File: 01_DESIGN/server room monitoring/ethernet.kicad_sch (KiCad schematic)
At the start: 38 parts, among them J6 HR911105A, U5 W5500, Y1 25 MHz

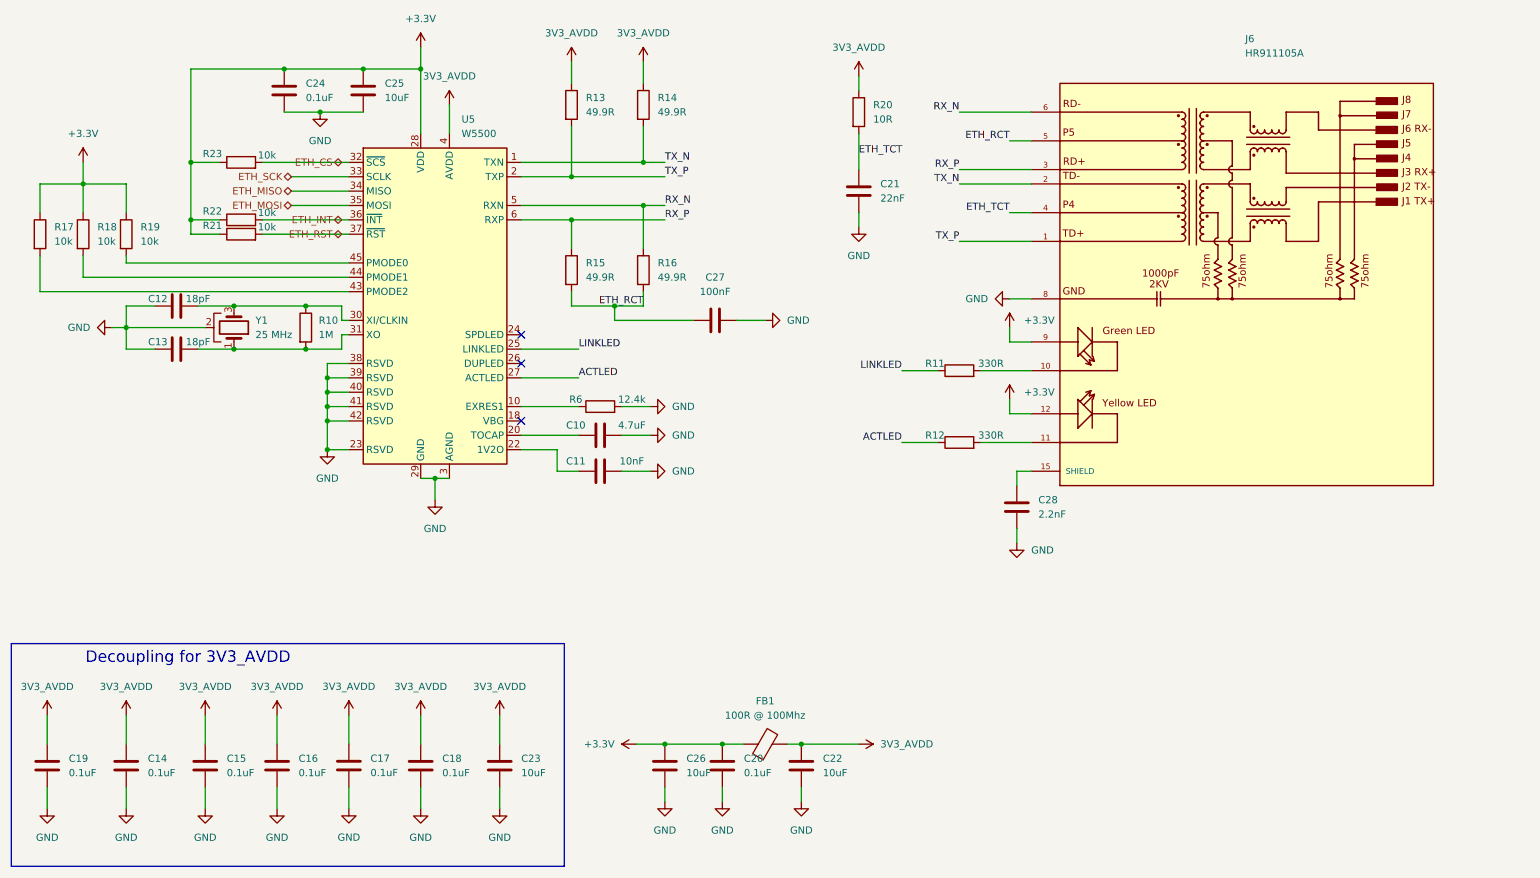
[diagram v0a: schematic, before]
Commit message: Update project files
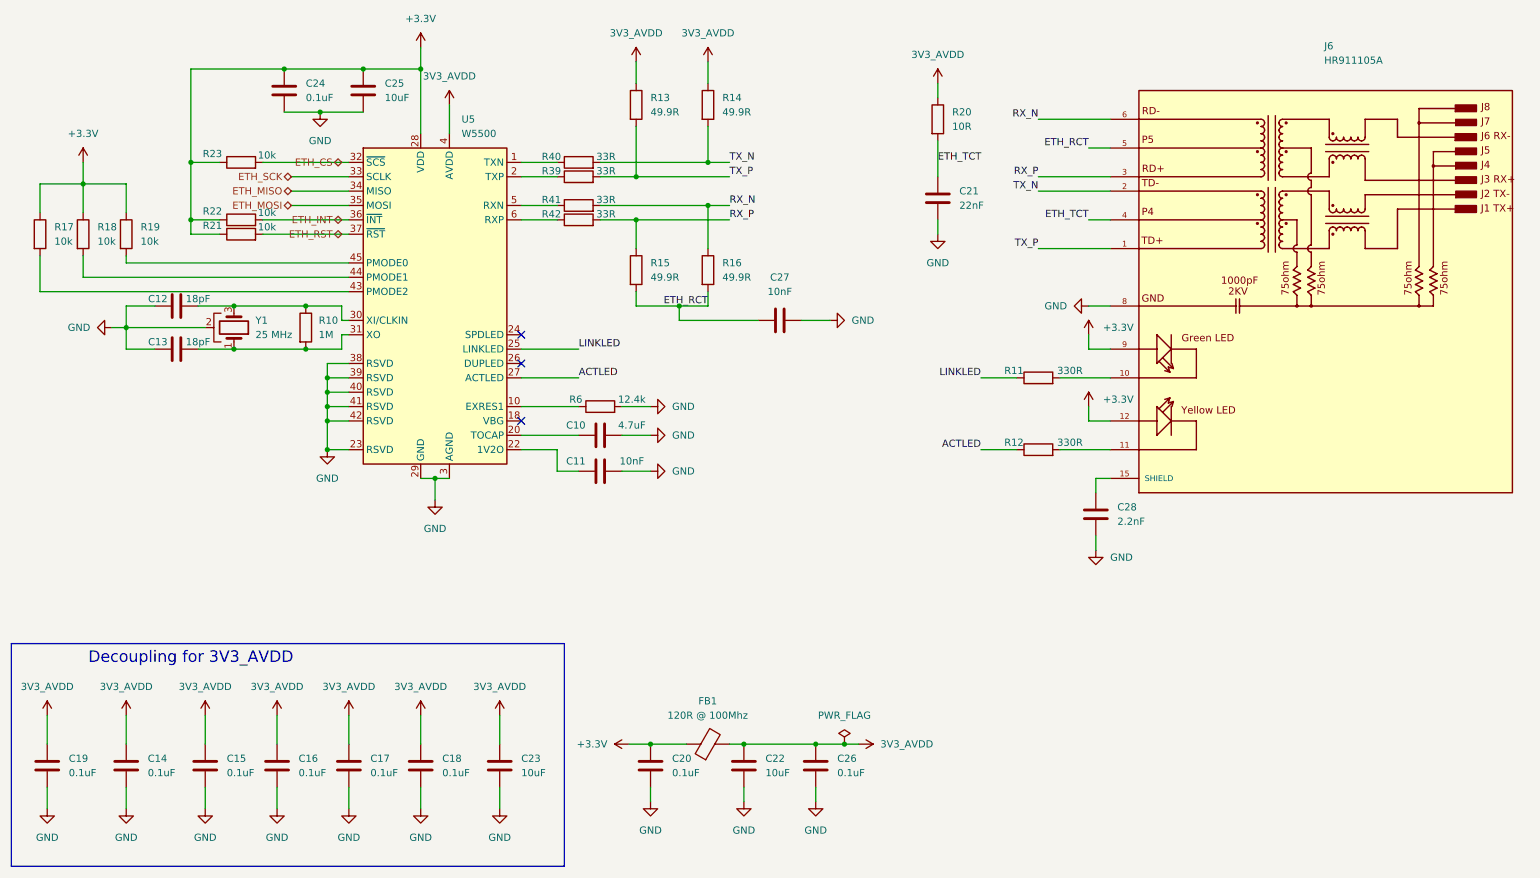
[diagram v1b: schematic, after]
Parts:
- added R39, R40, R41, R42: 33R, Resistor_SMD:R_0805_2012Metric, symbol Device:R
- C10, C11, C12, C13, C14, C15, C16, C17, C18, C19, C20, C21, C22, C23, C24, C25, C28: footprint CAP_C_3225X80 -> Capacitor_SMD:C_0805_2012Metric
- C26: value 10uF -> 0.1uF; footprint CAP_C_3225X80 -> Capacitor_SMD:C_0805_2012Metric
- C27: value 100nF -> 10nF; footprint CAP_C_3225X80 -> Capacitor_SMD:C_0805_2012Metric
- FB1: value 100R @ 100Mhz -> 120R @ 100Mhz
- R10, R11, R12, R13, R14, R15, R16, R17, R18, R19, R20, R21, R22, R23, R6: footprint RES_C_1005x30_L -> Resistor_SMD:R_0805_2012Metric
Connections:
- net +3.3V: no longer C26.1
- net 3V3_AVDD: now also C26.1
- net RX_N: now also R41.2; no longer U5.5 (RXN)
- net RX_P: now also R42.2; no longer U5.6 (RXP)
- net TX_N: now also R40.2; no longer U5.1 (TXN)
- net TX_P: now also R39.2; no longer U5.2 (TXP)
- new net: R39.1, U5.2 (TXP)
- new net: R40.1, U5.1 (TXN)
- new net: R41.1, U5.5 (RXN)
- new net: R42.1, U5.6 (RXP)
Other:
- moved on the sheet: C20, C21, C22, C27, C28, FB1, J6, R11, R12, R13, R14, R15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
